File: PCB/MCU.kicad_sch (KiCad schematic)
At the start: 23 parts, among them U4 STM32F051K6Ux, U5 INA180A3, Y1 8M

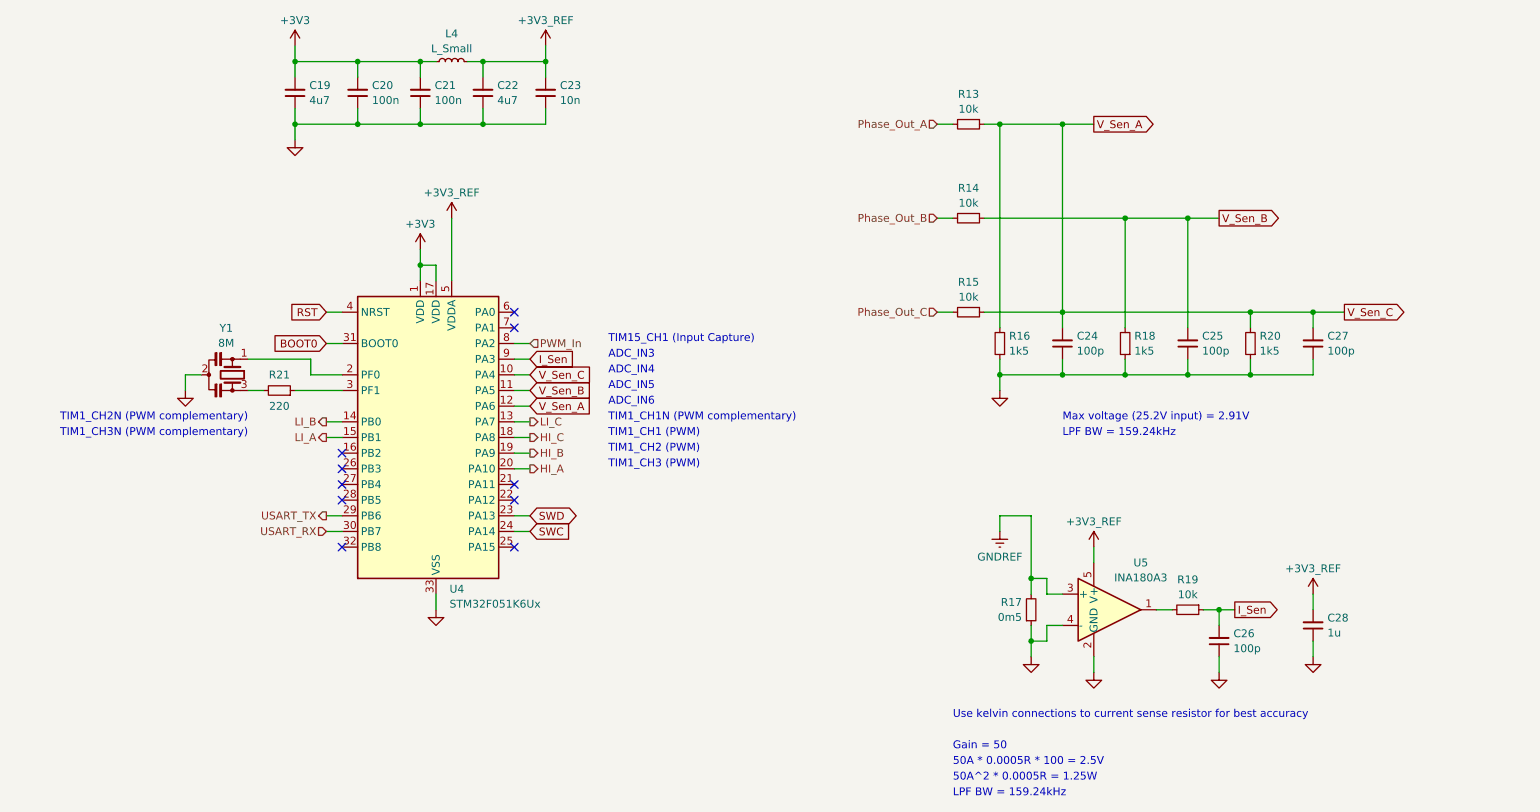
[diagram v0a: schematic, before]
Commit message: f
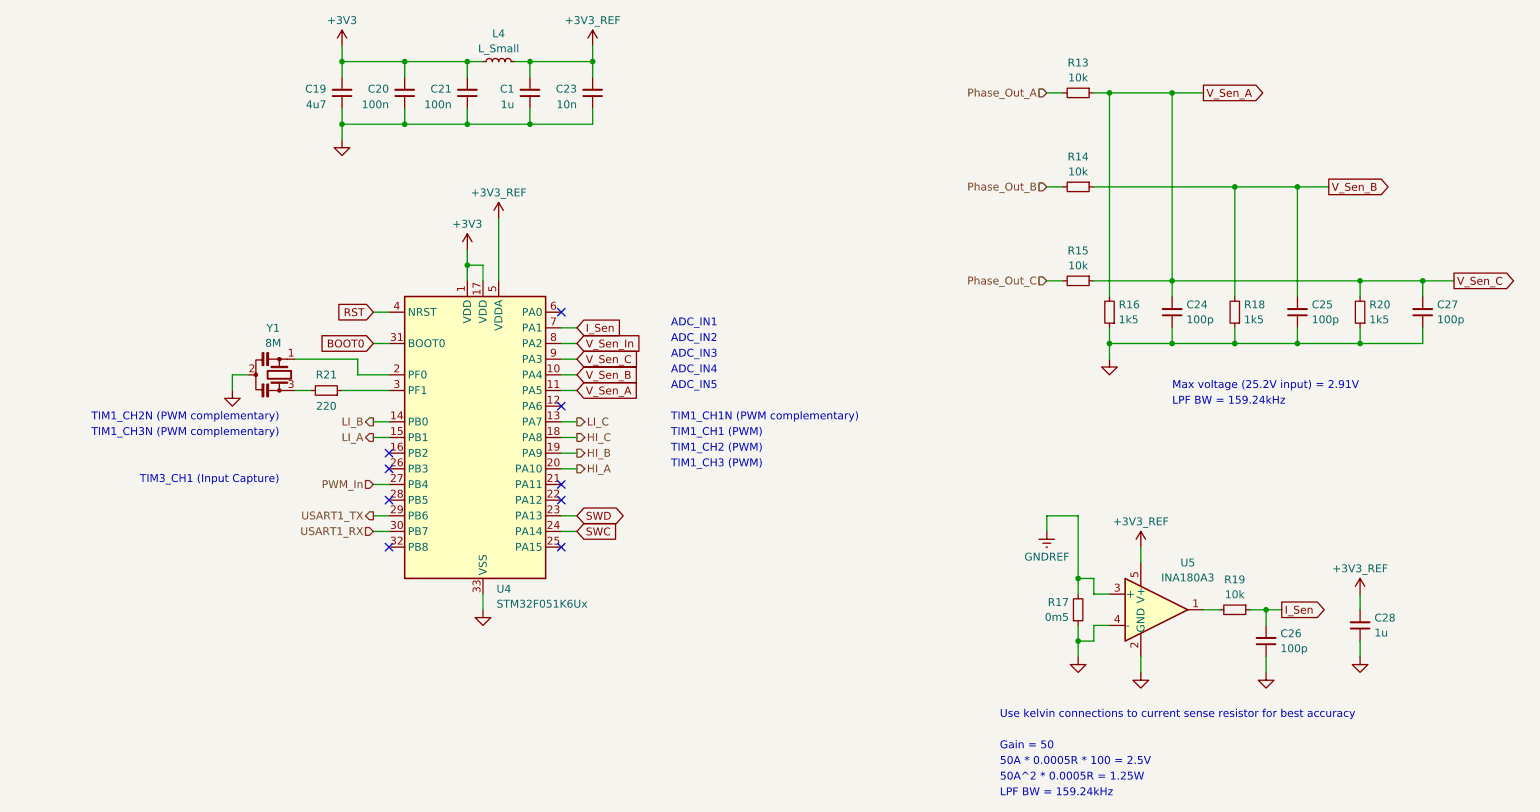
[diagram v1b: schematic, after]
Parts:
- removed C22: 4u7, Ariamelon-Device:C_0603_1608Metric, symbol Device:C_Small
- added C1: 1u, Ariamelon-Device:C_0603_1608Metric, symbol Device:C_Small
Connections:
- net +3V3_REF: now also C1.2
- net GND: now also C1.1
- net I_Sen: now also U4.7 (PA1); no longer U4.9 (PA3)
- net PWM_In: now also U4.27 (PB4); no longer U4.8 (PA2)
- net V_Sen_A: now also U4.11 (PA5), U4.9 (PA3); no longer U4.10 (PA4), U4.12 (PA6)
- net V_Sen_B: now also U4.10 (PA4); no longer U4.11 (PA5)
- net USART_RX renamed USART1_RX
- net USART_TX renamed USART1_TX
- new net V_Sen_In: U4.8 (PA2)
- no-connect marks 10 -> 9
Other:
- note added: "ADC_IN1"
- note added: "ADC_IN2"
- note added: "TIM3_CH1 (Input Capture)"
- note removed: "ADC_IN6"
- note removed: "TIM15_CH1 (Input Capture)"
- moved on the sheet: C19, C20, C21, C23, C24, C25, C26, C27, C28, L4, R13, R14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
